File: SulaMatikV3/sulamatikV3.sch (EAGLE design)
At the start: 29 parts, among them IC1 REG1117, IC2 74HC138N, Q3 2N5551

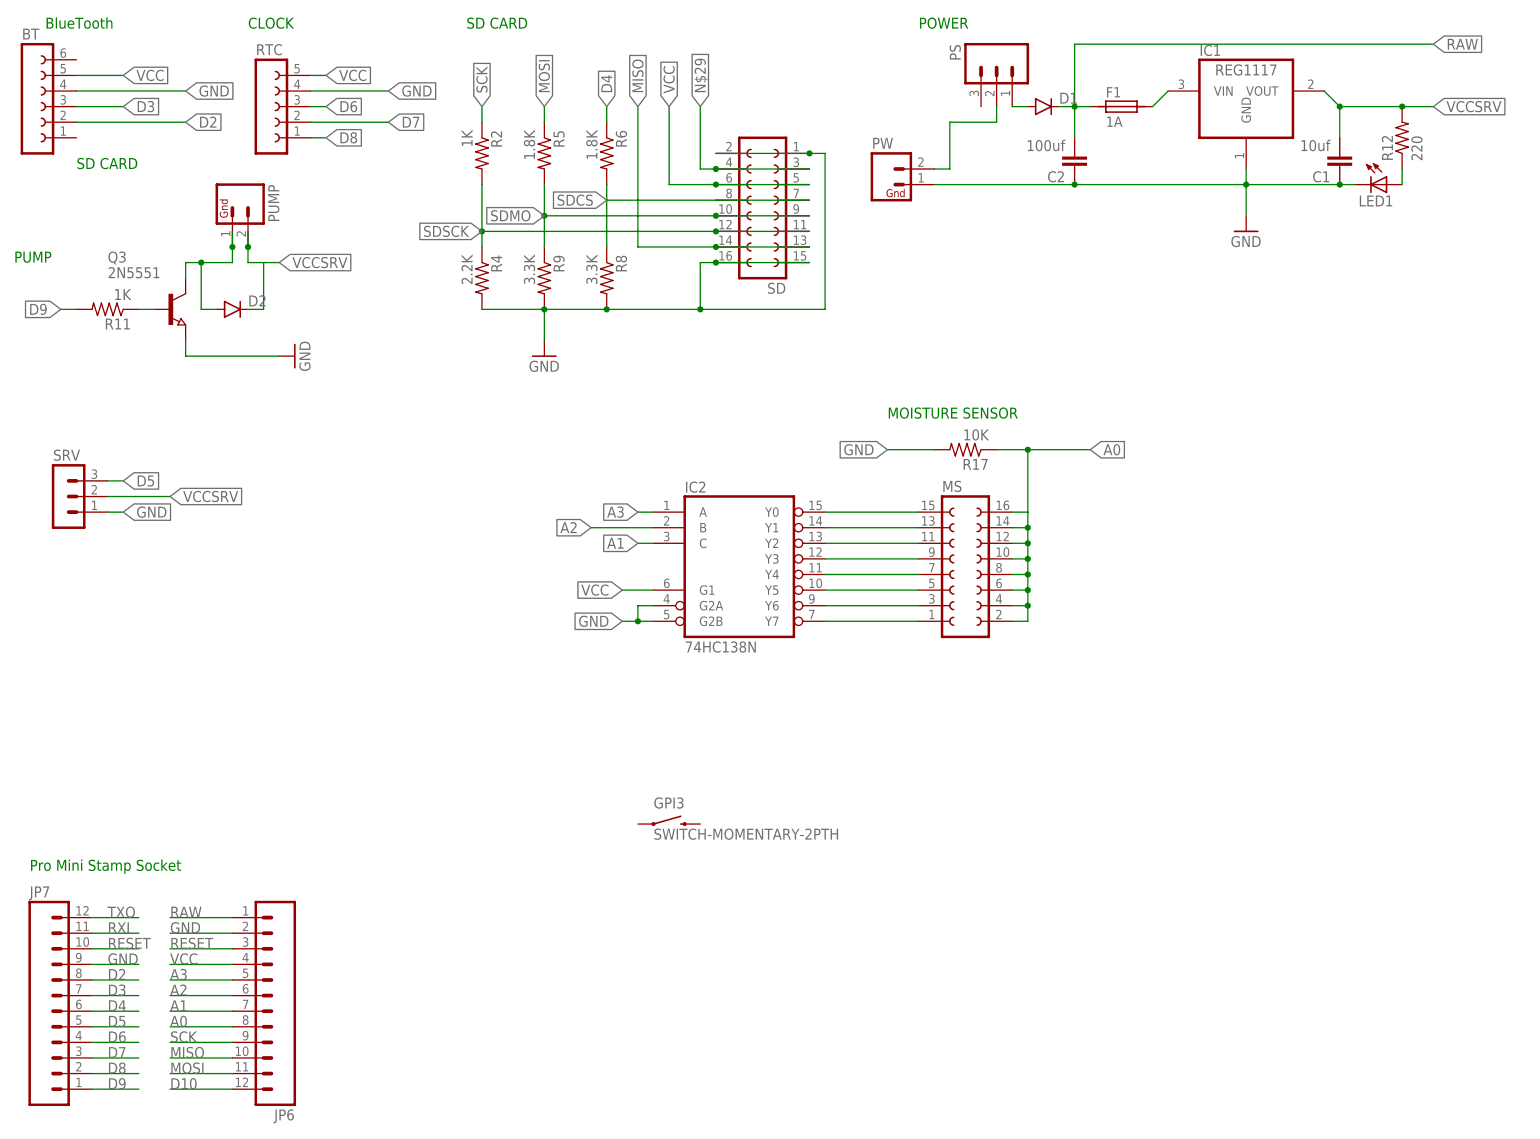
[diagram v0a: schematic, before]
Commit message: v3
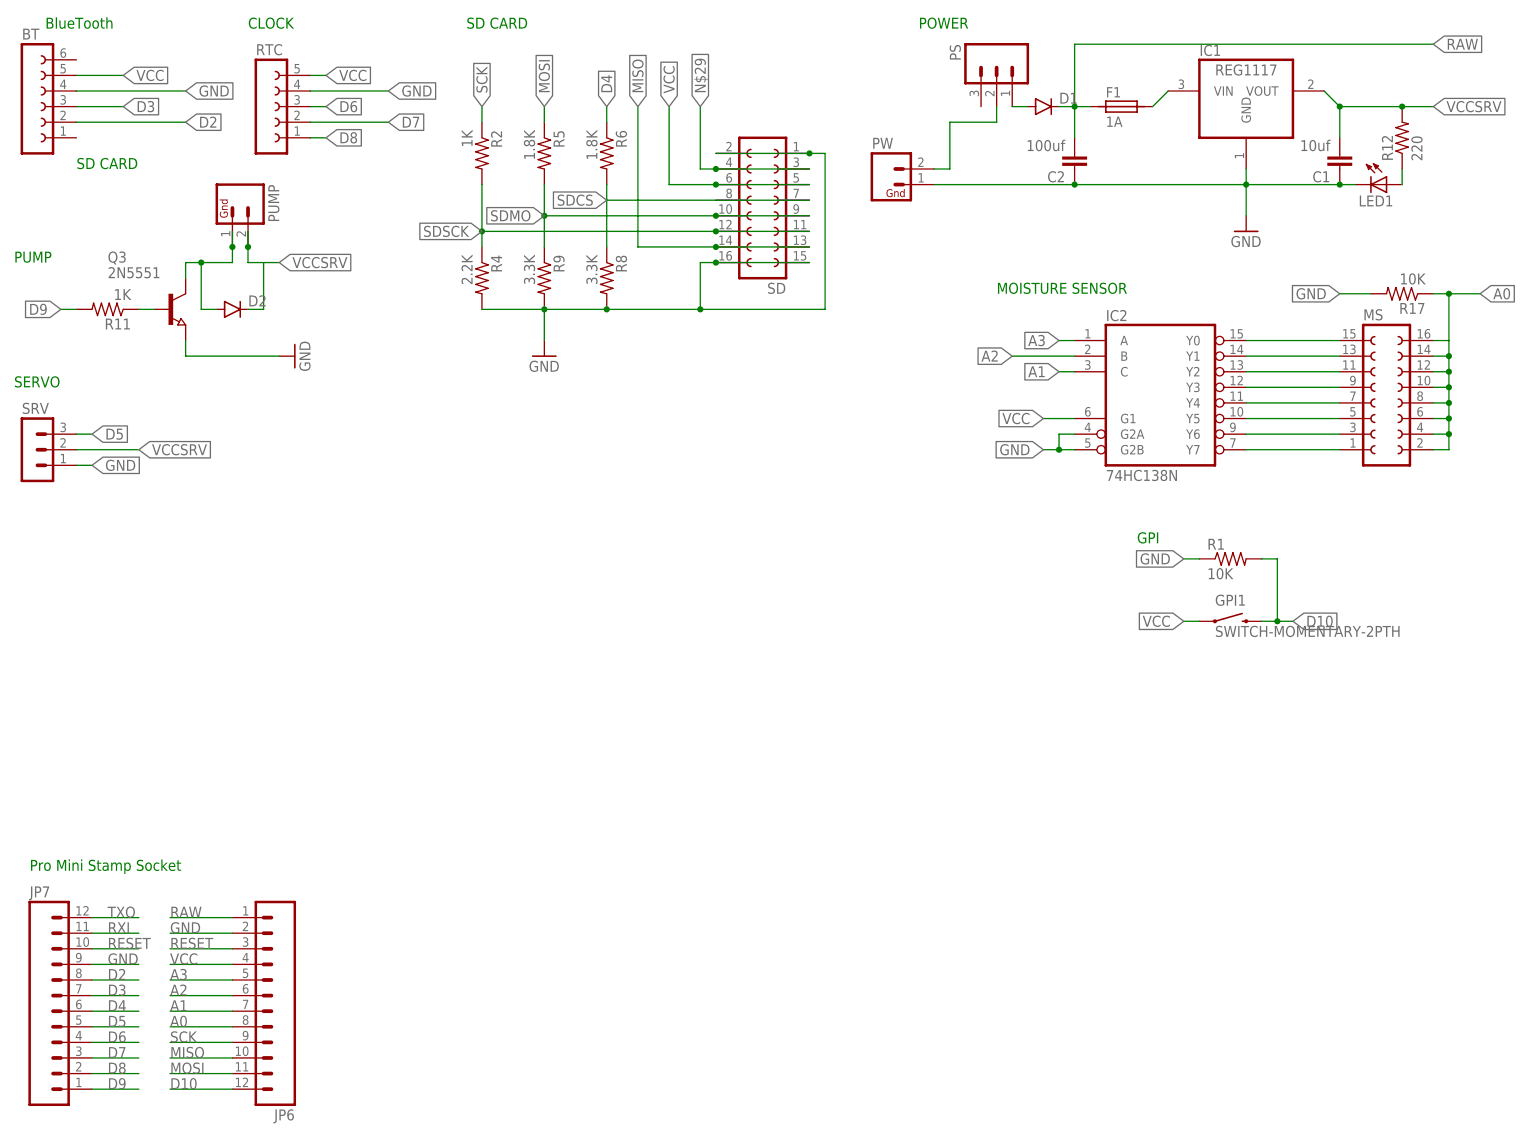
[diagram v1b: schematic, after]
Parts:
- removed GPI3: SWITCH-MOMENTARY-2PTH, SparkFun-Electromechanical:SWITCH-MOMENTARY-2PTH
- added GPI1: SWITCH-MOMENTARY-2PTH, SparkFun-Electromechanical:SWITCH-MOMENTARY-2PTH
- added R1: 10K, SparkFun-Passives:RESISTOR0805-RES
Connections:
- net D10: now also GPI1.2, R1.2
- net GND: now also R1.1
- net VCC: now also GPI1.1
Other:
- note added: "GPI"
- note added: "SERVO"
- moved on the sheet: IC2, MS, R17, SRV
